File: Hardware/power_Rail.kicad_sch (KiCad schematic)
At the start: 4 parts

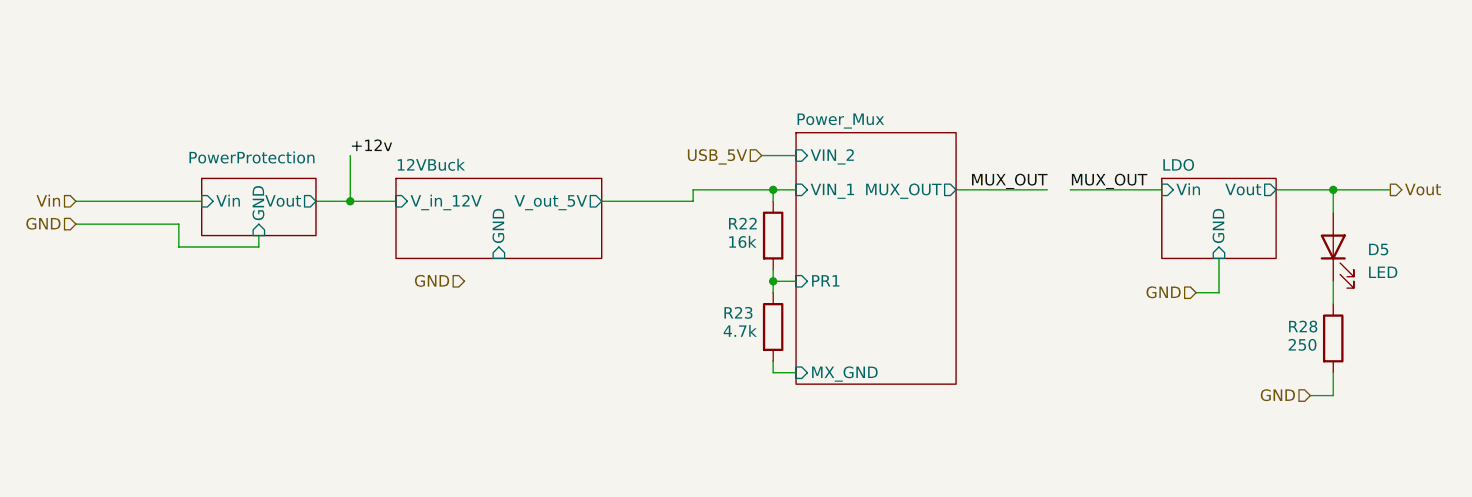
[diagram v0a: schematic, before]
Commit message: made review changes
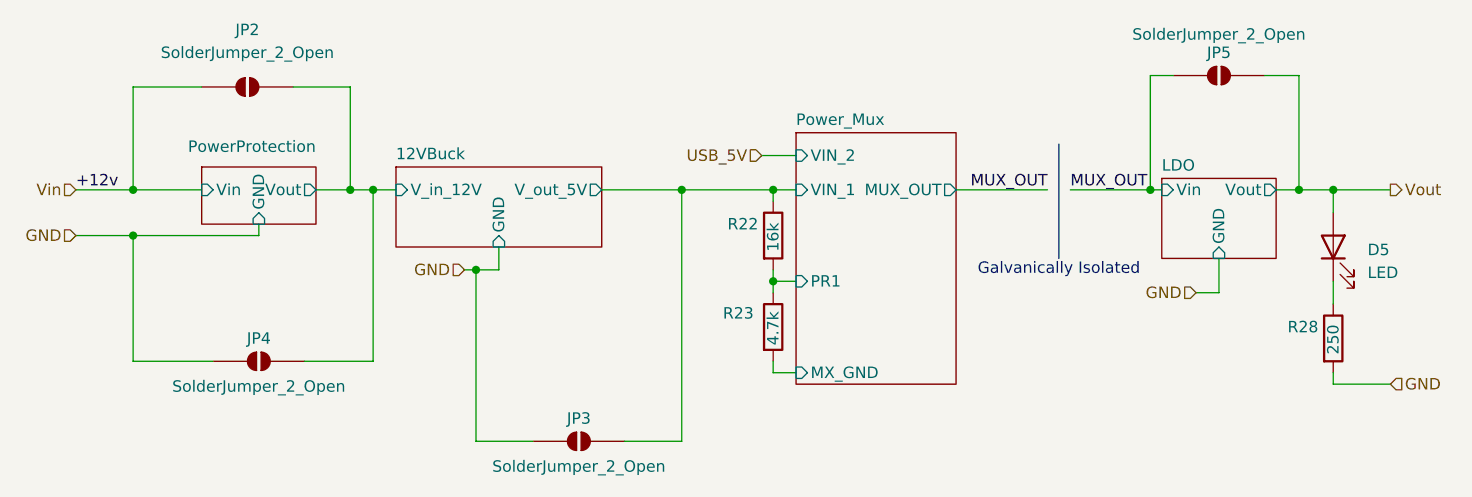
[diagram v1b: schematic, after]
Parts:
- added JP2, JP3, JP4, JP5: SolderJumper_2_Open, symbol Jumper:SolderJumper_2_Open
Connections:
- net 12VBuck/V_out_5V: now also JP3.2 (B)
- net GND: now also JP3.1 (A), JP4.1 (A)
- net MUX_OUT: now also JP5.1 (A)
- net Vin: now also JP2.1 (A)
- net Vout: now also JP5.2 (B)
- new net 12VBuck/V_in_12V: JP2.2 (B), JP4.2 (B)
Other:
- note added: "Galvanically Isolated"
